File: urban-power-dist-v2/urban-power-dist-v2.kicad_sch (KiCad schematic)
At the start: 24 parts, among them J1 ATF13-2P-BM03, J2 ATF13-2P-BM03, J3 ATF13-2P-BM03, J4 ATF13-2P-BM03

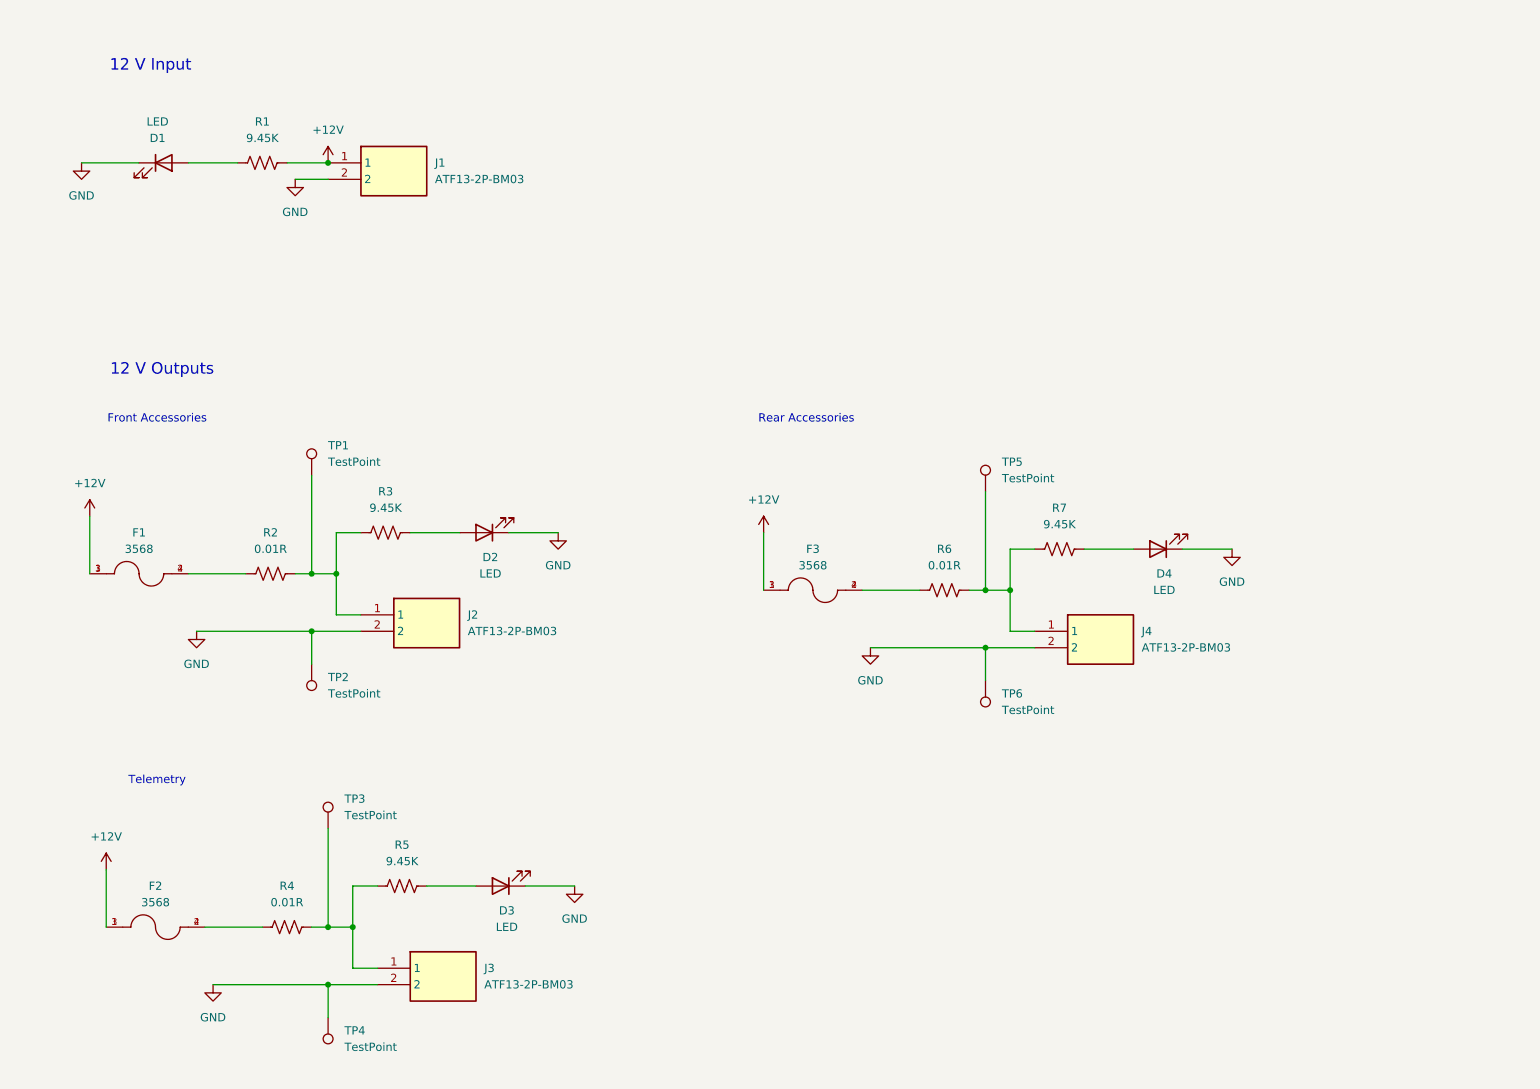
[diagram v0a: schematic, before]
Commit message: Revised schematic
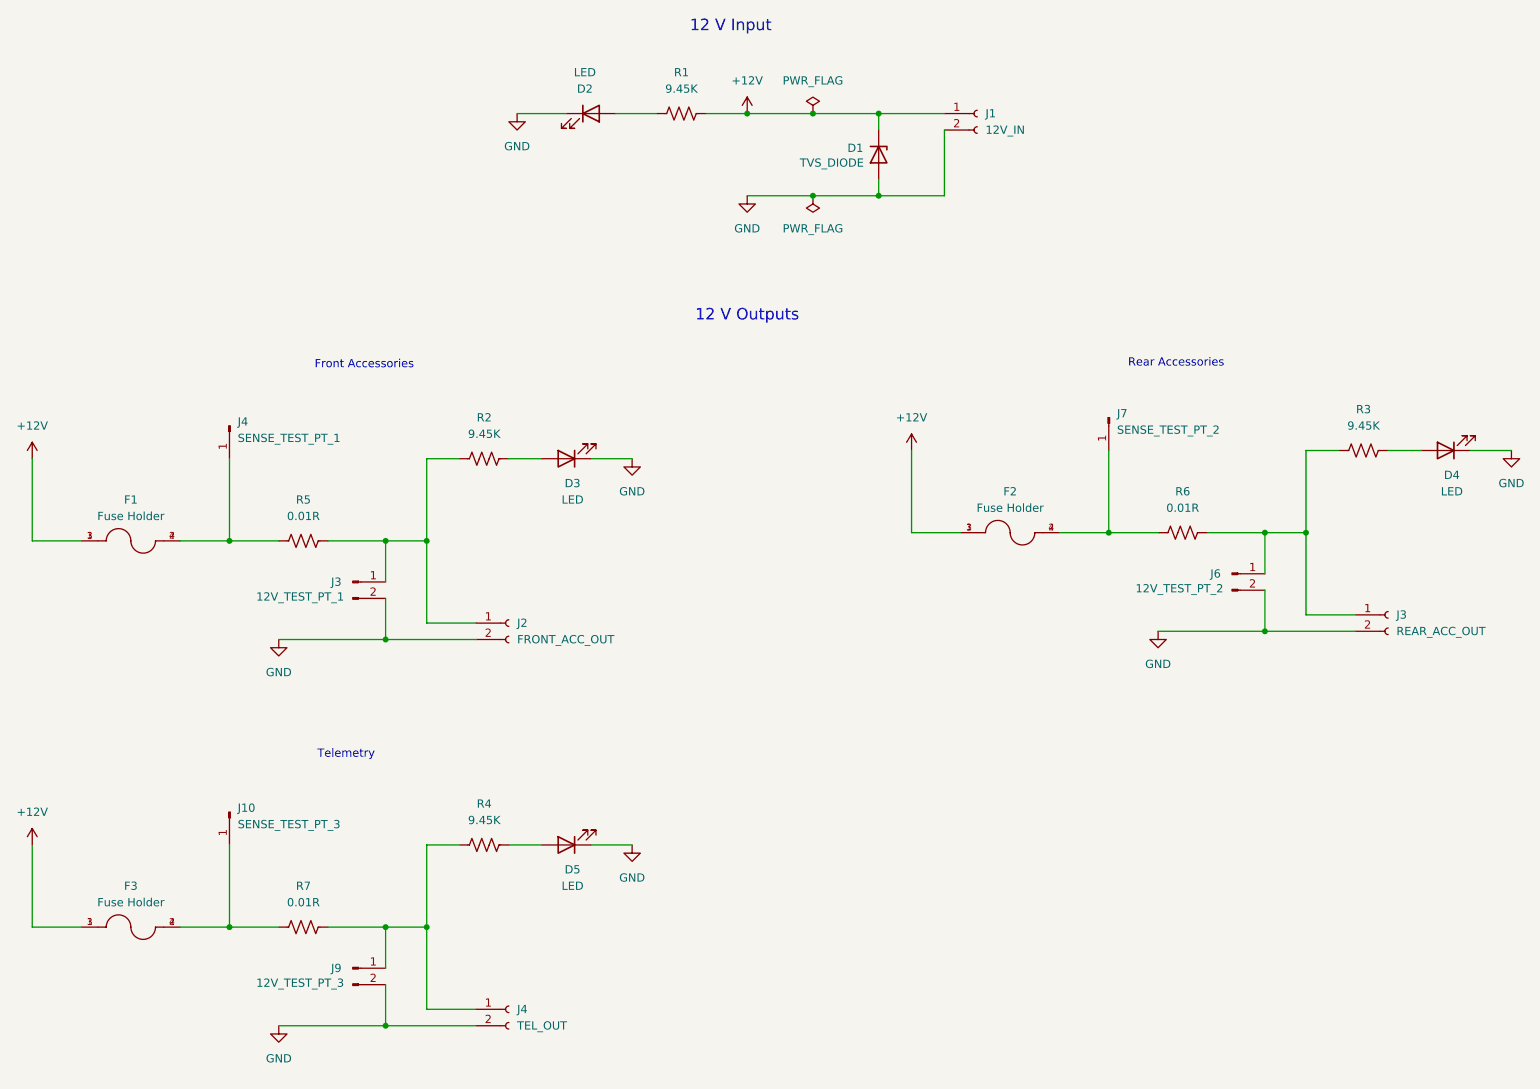
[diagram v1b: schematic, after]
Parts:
- removed D3: LED, LED_SMD:LED_0603_1608Metric_Pad1.05x0.95mm_HandSolder, symbol Device:LED
- removed J1, J2, J3, J4: ATF13-2P-BM03, ATF132PBM03, symbol ATF13-2P-BM03:ATF13-2P-BM03
- removed R5: 9.45K, Resistor_SMD:R_1206_3216Metric_Pad1.30x1.75mm_HandSolder, symbol Device:R_US
- removed TP1, TP2, TP3, TP4, TP5, TP6: TestPoint, symbol Connector:TestPoint
- added D1: TVS_DIODE, Diode_SMD:Nexperia_DSN1608-2_1.6x0.8mm, symbol Diode:PTVS12VZ1USK
- added D5: LED, LED_SMD:LED_0603_1608Metric_Pad1.05x0.95mm_HandSolder, symbol Device:LED
- added J1: 12V_IN, ATF13-2P-BM03:ATF132PBM03, symbol Connector:Conn_01x02_Socket
- added J10: SENSE_TEST_PT_3, Connector_PinHeader_2.54mm:PinHeader_1x01_P2.54mm_Vertical, symbol Connector:Conn_01x01_Pin
- added J2: FRONT_ACC_OUT, ATF13-2P-BM03:ATF132PBM03, symbol Connector:Conn_01x02_Socket
- added J3: 12V_TEST_PT_1, Connector_PinHeader_2.54mm:PinHeader_1x02_P2.54mm_Vertical, symbol Connector:Conn_01x02_Pin
- added J3: REAR_ACC_OUT, ATF13-2P-BM03:ATF132PBM03, symbol Connector:Conn_01x02_Socket
- added J4: TEL_OUT, ATF13-2P-BM03:ATF132PBM03, symbol Connector:Conn_01x02_Socket
- added J4: SENSE_TEST_PT_1, Connector_PinHeader_2.54mm:PinHeader_1x01_P2.54mm_Vertical, symbol Connector:Conn_01x01_Pin
- added J6: 12V_TEST_PT_2, Connector_PinHeader_2.54mm:PinHeader_1x02_P2.54mm_Vertical, symbol Connector:Conn_01x02_Pin
- added J7: SENSE_TEST_PT_2, Connector_PinHeader_2.54mm:PinHeader_1x01_P2.54mm_Vertical, symbol Connector:Conn_01x01_Pin
- added J9: 12V_TEST_PT_3, Connector_PinHeader_2.54mm:PinHeader_1x02_P2.54mm_Vertical, symbol Connector:Conn_01x02_Pin
- added R3: 9.45K, Resistor_SMD:R_1206_3216Metric_Pad1.30x1.75mm_HandSolder, symbol Device:R_US
- F1, F2, F3: value 3568 -> Fuse Holder
- R4: value 0.01R -> 9.45K; footprint Resistor_SMD:R_2512_6332Metric_Pad1.40x3.35mm_HandSolder -> Resistor_SMD:R_1206_3216Metric_Pad1.30x1.75mm_HandSolder
- R7: value 9.45K -> 0.01R; footprint Resistor_SMD:R_1206_3216Metric_Pad1.30x1.75mm_HandSolder -> Resistor_SMD:R_2512_6332Metric_Pad1.40x3.35mm_HandSolder
- renumbered D1 to D2, D2 to D3, R3 to R2, R2 to R5
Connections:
- net +12V: now also D1.1 (K), J1.1 (Pin_1)
- net GND: now also D1.2 (A), D5.1 (K), J1.2 (Pin_2), J2.2 (Pin_2), J3.2 (Pin_2), J3.2 (Pin_2), J4.2 (Pin_2), J6.2 (Pin_2), J9.2 (Pin_2)
- net at D4.2 (A): now also R3.1; no longer R7.1
- net at R6.2: now also J3.1 (Pin_1), J6.1 (Pin_1), R3.2; no longer R7.2
- net at F2.2, F2.4: now also R6.1, J7.1 (Pin_1); no longer R4.1
- net at F1.2, F1.4, R5.1: now also J4.1 (Pin_1)
- net at R2.2, R5.2: now also J2.1 (Pin_1), J3.1 (Pin_1)
- net at R4.2: now also R7.2, J4.1 (Pin_1), J9.1 (Pin_1)
- net at F3.2, F3.4: now also R7.1, J10.1 (Pin_1); no longer R6.1
- new net: D5.2 (A), R4.1
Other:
- moved on the sheet: D2, D3, F1, R1, R2, R5

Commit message: Revised schematic 2.0
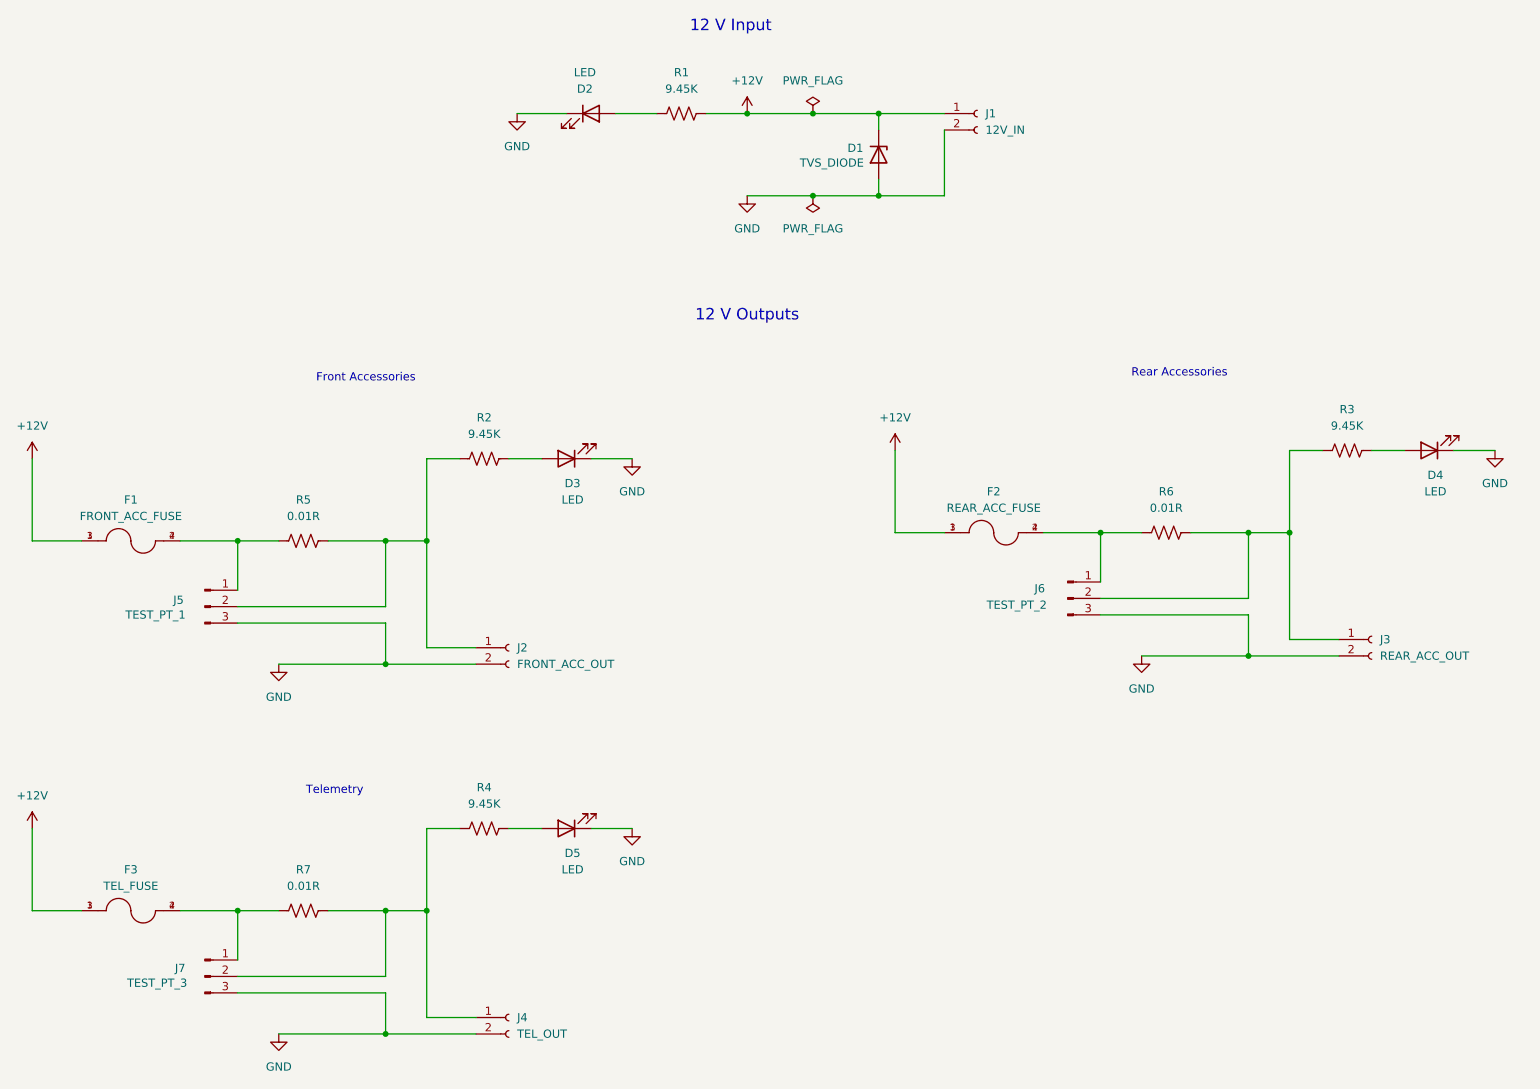
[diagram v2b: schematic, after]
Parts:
- removed J10: SENSE_TEST_PT_3, Connector_PinHeader_2.54mm:PinHeader_1x01_P2.54mm_Vertical, symbol Connector:Conn_01x01_Pin
- removed J3: 12V_TEST_PT_1, Connector_PinHeader_2.54mm:PinHeader_1x02_P2.54mm_Vertical, symbol Connector:Conn_01x02_Pin
- removed J4: SENSE_TEST_PT_1, Connector_PinHeader_2.54mm:PinHeader_1x01_P2.54mm_Vertical, symbol Connector:Conn_01x01_Pin
- removed J6: 12V_TEST_PT_2, Connector_PinHeader_2.54mm:PinHeader_1x02_P2.54mm_Vertical, symbol Connector:Conn_01x02_Pin
- removed J7: SENSE_TEST_PT_2, Connector_PinHeader_2.54mm:PinHeader_1x01_P2.54mm_Vertical, symbol Connector:Conn_01x01_Pin
- removed J9: 12V_TEST_PT_3, Connector_PinHeader_2.54mm:PinHeader_1x02_P2.54mm_Vertical, symbol Connector:Conn_01x02_Pin
- added J5: TEST_PT_1, Connector_PinHeader_2.54mm:PinHeader_1x03_P2.54mm_Vertical, symbol Connector:Conn_01x03_Pin
- added J6: TEST_PT_2, Connector_PinHeader_2.54mm:PinHeader_1x03_P2.54mm_Vertical, symbol Connector:Conn_01x03_Pin
- added J7: TEST_PT_3, Connector_PinHeader_2.54mm:PinHeader_1x03_P2.54mm_Vertical, symbol Connector:Conn_01x03_Pin
- F1: value Fuse Holder -> FRONT_ACC_FUSE
- F2: value Fuse Holder -> REAR_ACC_FUSE
- F3: value Fuse Holder -> TEL_FUSE
- R5, R6, R7: footprint Resistor_SMD:R_2512_6332Metric_Pad1.40x3.35mm_HandSolder -> Resistor_SMD:R_0805_2012Metric_Pad1.20x1.40mm_HandSolder
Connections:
- net GND: now also J5.3 (Pin_3), J6.3 (Pin_3), J7.3 (Pin_3)
- net at J3.1 (Pin_1), R3.2, R6.2: now also J6.2 (Pin_2)
- net at J2.1 (Pin_1), R2.2, R5.2: now also J5.2 (Pin_2)
- net at F1.2, F1.4, R5.1: now also J5.1 (Pin_1)
- net at J4.1 (Pin_1), R4.2, R7.2: now also J7.2 (Pin_2)
- net at F3.2, F3.4, R7.1: now also J7.1 (Pin_1)
- net at F2.2, F2.4, R6.1: now also J6.1 (Pin_1)
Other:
- moved on the sheet: J2

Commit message: Revised schematic 3.0
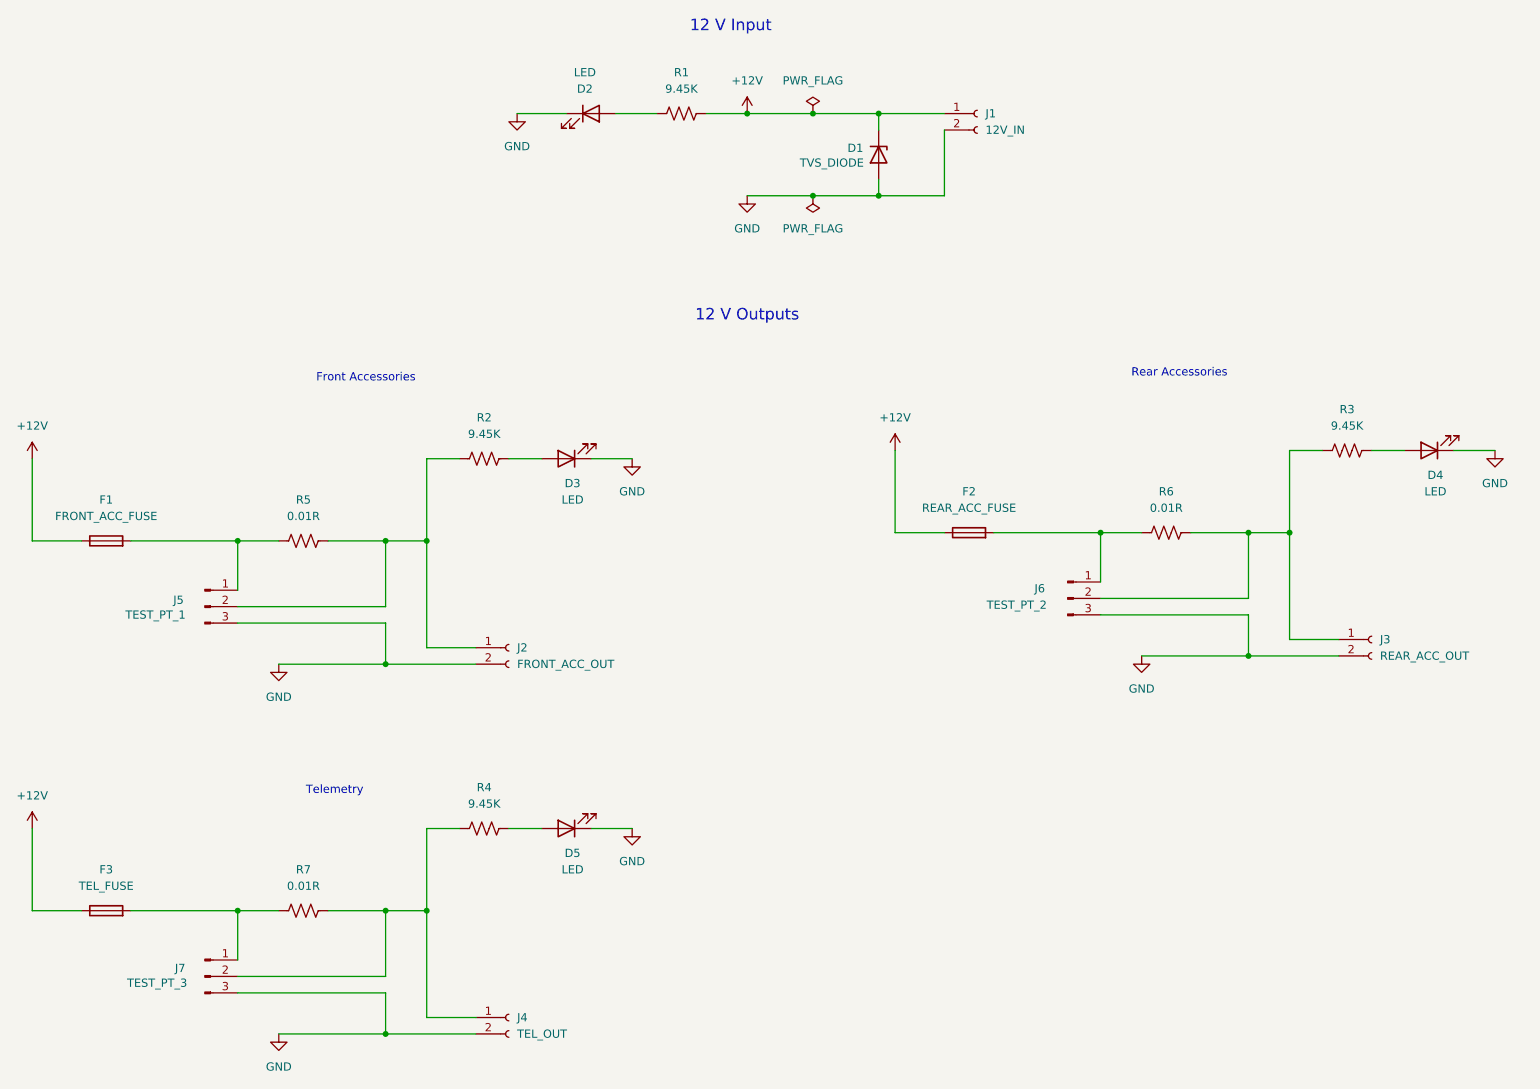
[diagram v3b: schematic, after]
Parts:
- removed F1: FRONT_ACC_FUSE, 3568:FUSE_3568, symbol 3568:3568
- removed F2: REAR_ACC_FUSE, 3568:FUSE_3568, symbol 3568:3568
- removed F3: TEL_FUSE, 3568:FUSE_3568, symbol 3568:3568
- added F1: FRONT_ACC_FUSE, Fuse:Fuseholder_Blade_Mini_Keystone_3568, symbol Device:Fuse
- added F2: REAR_ACC_FUSE, Fuse:Fuseholder_Blade_Mini_Keystone_3568, symbol Device:Fuse
- added F3: TEL_FUSE, Fuse:Fuseholder_Blade_Mini_Keystone_3568, symbol Device:Fuse
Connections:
- net +12V: now also F1.1, F2.1, F3.1
- net at J6.1 (Pin_1), R6.1: now also F2.2
- net at J7.1 (Pin_1), R7.1: now also F3.2
- net at J5.1 (Pin_1), R5.1: now also F1.2
